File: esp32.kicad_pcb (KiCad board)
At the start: 2 copper layers, 43.2 x 65 mm, 26 parts, among them J1 USB_C_Receptacle, SW1 SW_SPST, SW2 SW_SPST, U1 ESP32-S3-WROOM-1, U3 AMS1117-3.3, U5 TPD2EUSB30A

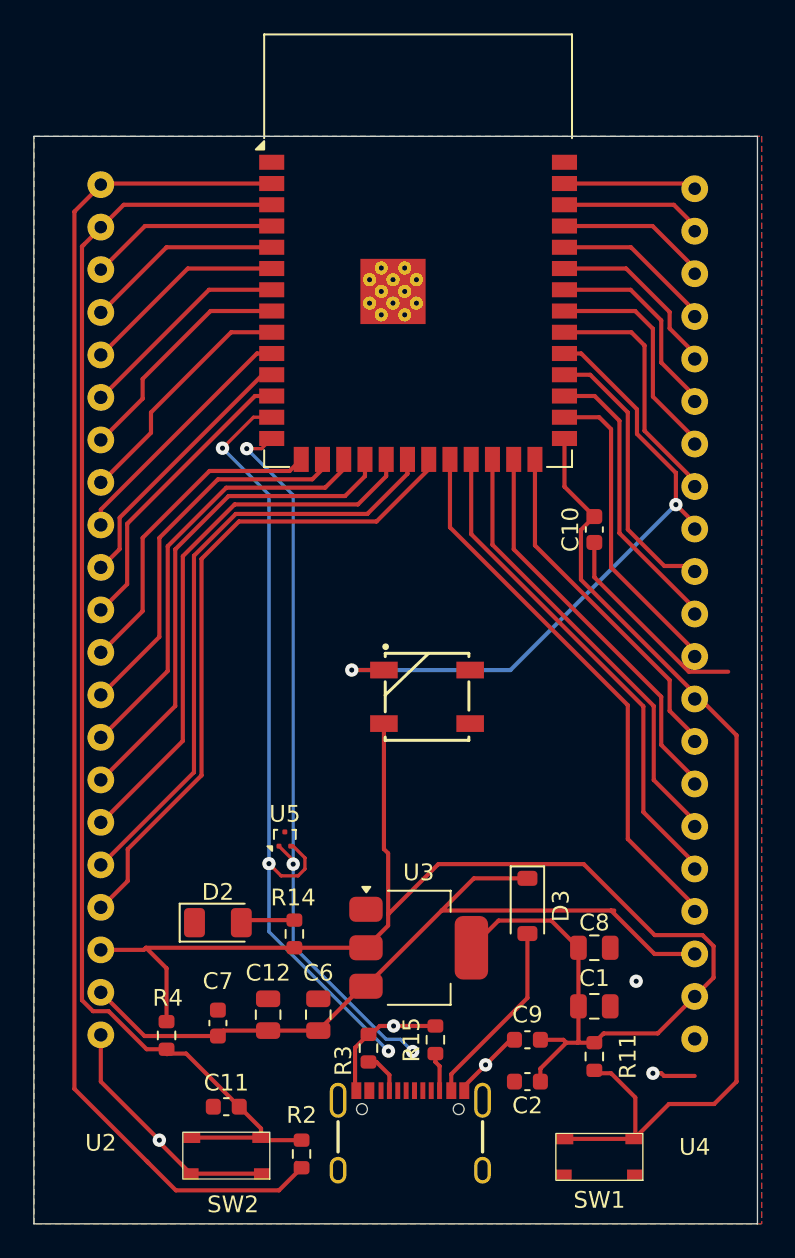
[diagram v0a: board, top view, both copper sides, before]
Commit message: Reference board
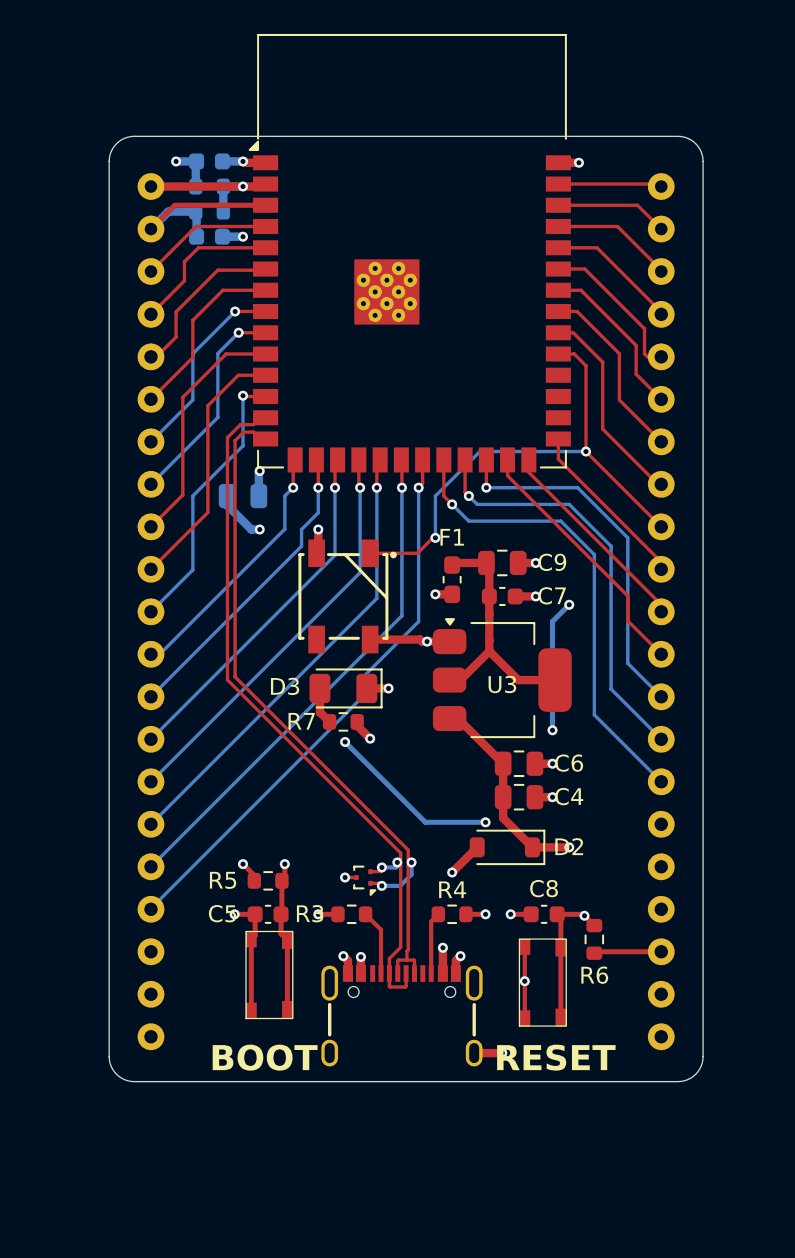
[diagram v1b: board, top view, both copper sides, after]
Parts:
- removed C12: 10u, Capacitor_SMD:C_0805_2012Metric
- removed the C8 at (160.0, 103.5)
- added C3: 1u, Capacitor_SMD:C_0603_1608Metric, B.Cu at (137.0, 61.0)
- added C6: 100n, Capacitor_SMD:C_0805_2012Metric, F.Cu at (155.5, 92.5)
- added F1: 500mA, Fuse:Fuse_0603_1608Metric_Pad1.05x0.95mm_HandSolder, F.Cu at (151.5, 81.5)
- added R1: 0, Resistor_SMD:R_0603_1608Metric, B.Cu at (137.0, 58.0)
- C1, C2, R2: moved to B.Cu
- C7: value 0.1u -> 100n
- C9: value 0.1u -> 10u; footprint Capacitor_SMD:C_0603_1608Metric -> Capacitor_SMD:C_0805_2012Metric
- moved C2 58.2 mm to (137.0, 56.5), turned to 0 degrees
- moved R2 56.6 mm to (137.0, 59.5), turned to 180 degrees
- moved C1 37.0 mm to (139.0, 76.5), turned to 180 degrees
- moved C7 30.6 mm to (154.5, 82.5), turned to 0 degrees
- moved C5 30.2 mm to (140.5, 101.5), turned to 0 degrees
- moved C9 28.5 mm to (154.5, 80.5)
- moved R6 26.2 mm to (160.0, 103.0), turned to 90 degrees
- moved SW2 24.3 mm to (161.9, 105.8), turned to 90 degrees
- moved C8 22.2 mm to (157.0, 101.5)
- moved R5 22.1 mm to (140.5, 99.5), turned to 0 degrees
- moved C4 17.7 mm to (155.5, 94.5), turned to 0 degrees
- moved U3 16.8 mm to (154.5, 87.5)
- moved SW1 16.0 mm to (145.6, 105.3), turned to 90 degrees
- moved D3 15.9 mm to (145.0, 88.0), turned to 180 degrees
- moved R7 13.0 mm to (145.0, 90.0), turned to 180 degrees
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- renumbered C6 to C4, C10 to C5, C11 to C8, D3 to D2, D2 to D3, R15 to R4, R11 to R5, R4 to R6, R14 to R7, U5 to U2, U2 to U4, U4 to U5
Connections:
- net /USB_DN renamed /USB_D-
- net /USB_DP renamed /USB_D+
- net ESP_3V3 renamed +ESP_3V3
- C7 pad 1: +5V -> /3V3_preFuse
- C9 pad 1: GND -> /3V3_preFuse
- C9 pad 2: +3V3 -> GND
- U1 pad 28: /GPIO35 -> unconnected-(U1-IO35-Pad28)
- U1 pad 29: /GPIO36 -> unconnected-(U1-IO36-Pad29)
- U1 pad 30: /GPIO37 -> unconnected-(U1-IO37-Pad30)
- U3 pad 2: +3V3 -> /3V3_preFuse
- U5 pad 10: /GPIO37 -> /GPIO0
- U5 pad 11: /GPIO36 -> /GPIO45
- U5 pad 12: /GPIO35 -> /GPIO48
- U5 pad 13: /GPIO0 -> /GPIO47
- U5 pad 14: /GPIO45 -> /GPIO21
- U5 pad 15: /GPIO48 -> /GPIO14
- U5 pad 16: /GPIO47 -> unconnected-(U5-Pad16)
- U5 pad 17: /GPIO21 -> unconnected-(U5-Pad17)
- U5 pad 18: /GPIO14 -> unconnected-(U5-Pad18)
- U5 pad 19: +5V -> +3V3
- U5 pad 20: +3V3 -> +5V
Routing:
- net +ESP_3V3: track 82.1 -> 9.80 mm, vias 0 -> 1
- net +3V3: track 87.9 -> 106.6 mm, vias 0 -> 6
- net /GPIO35: track 18.4 -> 0.00 mm
- net /GPIO36: track 17.0 -> 0.00 mm
- net /GPIO37: track 16.6 -> 0.00 mm
- net /3V3_preFuse: track 0.00 -> 15.2 mm
- net /GPIO38: track 39.4 -> 30.3 mm
- net /GPIO45: track 20.5 -> 12.4 mm
- net /GPIO48: track 23.6 -> 15.4 mm
- net /GPIO0: track 60.8 -> 52.9 mm, vias 0 -> 3
- net +5V: track 46.9 -> 53.7 mm, vias 0 -> 1
- net /GPIO12: track 36.5 -> 30.5 mm, vias 0 -> 1
- net /GPIO11: track 33.1 -> 27.5 mm, vias 0 -> 1
- net /GPIO13: track 39.2 -> 33.6 mm, vias 0 -> 1
- net /GPIO10: track 29.8 -> 24.4 mm, vias 0 -> 1
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- added copper zone on In1.Cu, net GND
- removed copper zone on B.Cu, net GND
- removed copper zone on F.Cu, net GND
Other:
- board size 43.2 x 65 mm -> 35.5 x 56.5 mm
- copper layers 2 -> 4
- board text added: "BOOT"
- board text added: "RESET"
